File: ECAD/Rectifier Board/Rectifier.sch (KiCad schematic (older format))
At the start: 3 parts

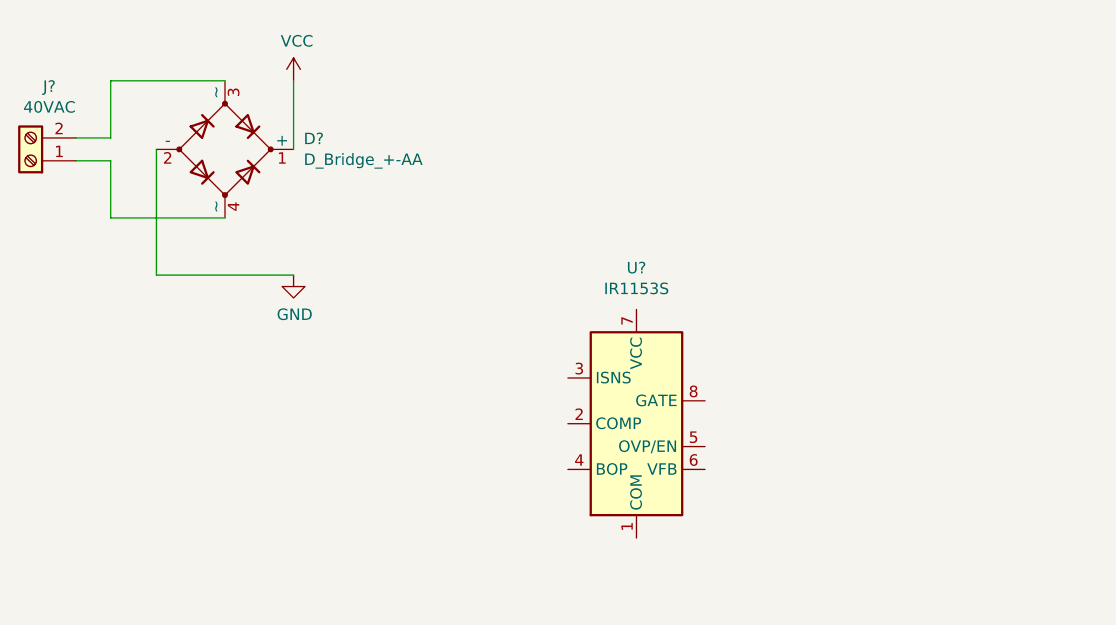
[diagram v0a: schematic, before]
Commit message: rectifier
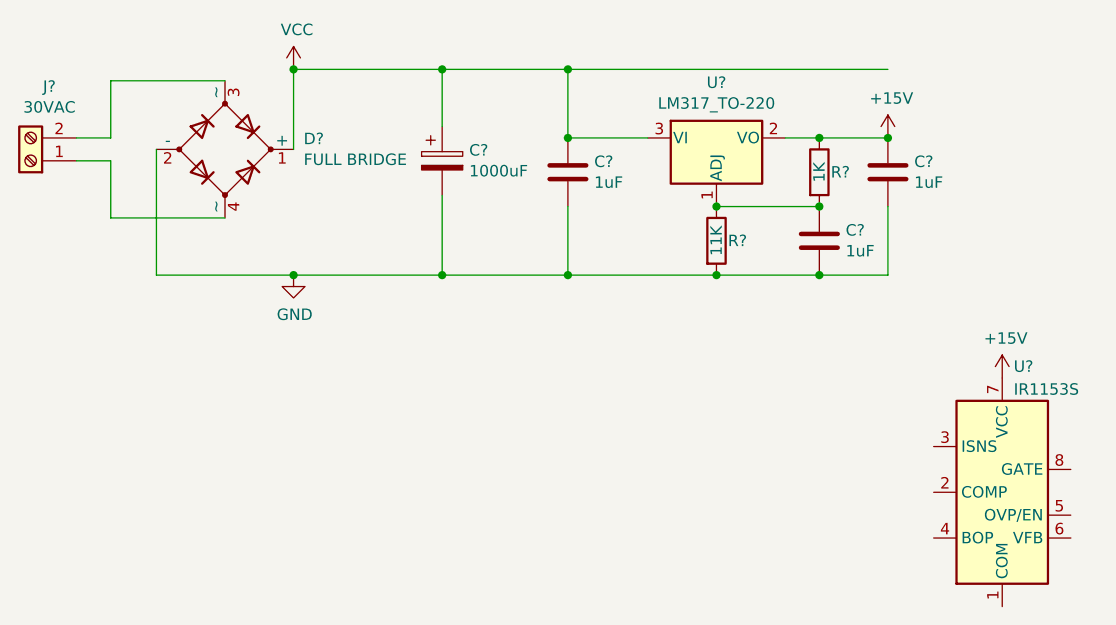
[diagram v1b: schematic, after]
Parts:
- added C? (x3): 1uF, symbol Device:C
- added C?: 1000uF, symbol Device:CP
- added R?: 11K, symbol Device:R
- added R?: 1K, symbol Device:R
- added U?: LM317_TO-220, Package_TO_SOT_THT:TO-220-3_Vertical, symbol Regulator_Linear:LM317_TO-220
- D?: value D_Bridge_+-AA -> FULL BRIDGE
- J?: value 40VAC -> 30VAC
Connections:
- net labels added: +15V
- wire segments 9 -> 26
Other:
- moved on the sheet: U?
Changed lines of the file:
@@
 P 3000 2950
 F 0 "D?" H 3344 2996 50  0000 L CNN
-F 1 "D_Bridge_+-AA" H 3344 2905 50  0000 L CNN
+F 1 "FULL BRIDGE" H 3344 2905 50  0000 L CNN
 F 2 "" H 3000 2950 50  0001 C CNN
 F 3 "~" H 3000 2950 50  0001 C CNN
@@
 L Regulator_Controller:IR1153S U?
 U 1 1 62058102
-P 4800 4150
-F 0 "U?" H 4800 4831 50  0000 C CNN
-F 1 "IR1153S" H 4800 4740 50  0000 C CNN
-F 2 "Package_SO:SOIC-8_3.9x4.9mm_P1.27mm" H 4800 4150 50  0001 C CIN
-F 3 "https://www.infineon.com/dgdl/ir1153.pdf?fileId=5546d462533600a4015355c42a5b1649" H 4800 4150 50  0001 C CNN
-	1    4800 4150
+P 6400 4450
+F 0 "U?" H 6450 5000 50  0000 L CNN
+F 1 "IR1153S" H 6450 4900 50  0000 L CNN
+F 2 "Package_SO:SOIC-8_3.9x4.9mm_P1.27mm" H 6400 4450 50  0001 C CIN
+F 3 "https://www.infineon.com/dgdl/ir1153.pdf?fileId=5546d462533600a4015355c42a5b1649" H 6400 4450 50  0001 C CNN
+	1    6400 4450
 	1    0    0    -1
 $EndComp
@@
 P 2150 3000
 F 0 "J?" H 2068 2675 50  0000 C CNN
-F 1 "40VAC" H 2068 2766 50  0000 C CNN
+F 1 "30VAC" H 2068 2766 50  0000 C CNN
 F 2 "" H 2150 3000 50  0001 C CNN
 F 3 "~" H 2150 3000 50  0001 C CNN
@@
 Wire Wire Line
 	2700 3500 3300 3500
-Wire Wire Line
-	3300 2950 3300 2650
 $Comp
 L power:VCC #PWR?
 U 1 1 6205AED4
-P 3300 2650
-F 0 "#PWR?" H 3300 2500 50  0001 C CNN
-F 1 "VCC" H 3315 2823 50  0000 C CNN
-F 2 "" H 3300 2650 50  0001 C CNN
-F 3 "" H 3300 2650 50  0001 C CNN
-	1    3300 2650
-	1    0    0    -1
-$EndComp
+P 3300 2600
+F 0 "#PWR?" H 3300 2450 50  0001 C CNN
+F 1 "VCC" H 3315 2773 50  0000 C CNN
+F 2 "" H 3300 2600 50  0001 C CNN
+F 3 "" H 3300 2600 50  0001 C CNN
+	1    3300 2600
+	1    0    0    -1
+$EndComp
+$Comp
+L Regulator_Linear:LM317_TO-220 U?
+U 1 1 6205D4E8
+P 5150 2900
+F 0 "U?" H 5150 3142 50  0000 C CNN
+F 1 "LM317_TO-220" H 5150 3051 50  0000 C CNN
+F 2 "Package_TO_SOT_THT:TO-220-3_Vertical" H 5150 3150 50  0001 C CIN
+F 3 "http://www.ti.com/lit/ds/symlink/lm317.pdf" H 5150 2900 50  0001 C CNN
+	1    5150 2900
+	1    0    0    -1
+$EndComp
+$Comp
+L Device:R R?
+U 1 1 6205E083
+P 5150 3350
+F 0 "R?" H 5200 3350 50  0000 L CNN
+F 1 "11K" V 5150 3350 50  0000 C CNN
+F 2 "" V 5080 3350 50  0001 C CNN
+F 3 "~" H 5150 3350 50  0001 C CNN
+	1    5150 3350
+	1    0    0    -1
+$EndComp
+$Comp
+L Device:R R?
+U 1 1 6205F378
+P 5600 3050
+F 0 "R?" H 5650 3050 50  0000 L CNN
+F 1 "1K" V 5600 3050 50  0000 C CNN
+F 2 "" V 5530 3050 50  0001 C CNN
+F 3 "~" H 5600 3050 50  0001 C CNN
+	1    5600 3050
+	1    0    0    -1
+$EndComp
+Wire Wire Line
+	5150 3200 5600 3200
+Connection ~ 5150 3200
+Wire Wire Line
+	5600 2900 5450 2900
+$Comp
+L Device:C C?
+U 1 1 6205FE8A
+P 5900 3050
+F 0 "C?" H 6015 3096 50  0000 L CNN
+F 1 "1uF" H 6015 3005 50  0000 L CNN
+F 2 "" H 5938 2900 50  0001 C CNN
+F 3 "~" H 5900 3050 50  0001 C CNN
+	1    5900 3050
+	1    0    0    -1
+$EndComp
+$Comp
+L Device:C C?
+U 1 1 620613FC
+P 5600 3350
+F 0 "C?" H 5715 3396 50  0000 L CNN
+F 1 "1uF" H 5715 3305 50  0000 L CNN
+F 2 "" H 5638 3200 50  0001 C CNN
+F 3 "~" H 5600 3350 50  0001 C CNN
+	1    5600 3350
+	1    0    0    -1
+$EndComp
+Connection ~ 5600 3200
+Wire Wire Line
+	5150 3500 5600 3500
+Wire Wire Line
+	5600 3500 5900 3500
+Wire Wire Line
+	5900 3500 5900 3200
+Connection ~ 5600 3500
+Wire Wire Line
+	5900 2900 5600 2900
+Connection ~ 5600 2900
+$Comp
+L Device:C C?
+U 1 1 620625CD
+P 4500 3050
+F 0 "C?" H 4615 3096 50  0000 L CNN
+F 1 "1uF" H 4615 3005 50  0000 L CNN
+F 2 "" H 4538 2900 50  0001 C CNN
+F 3 "~" H 4500 3050 50  0001 C CNN
+	1    4500 3050
+	1    0    0    -1
+$EndComp
+Wire Wire Line
+	4500 3500 4500 3200
+Wire Wire Line
+	4850 2900 4500 2900
+Wire Wire Line
+	4500 3500 5150 3500
+Connection ~ 5150 3500
+$Comp
+L Device:CP C?
+U 1 1 62063BAE
+P 3950 3000
+F 0 "C?" H 4068 3046 50  0000 L CNN
+F 1 "1000uF" H 4068 2955 50  0000 L CNN
+F 2 "" H 3988 2850 50  0001 C CNN
+F 3 "~" H 3950 3000 50  0001 C CNN
+	1    3950 3000
+	1    0    0    -1
+$EndComp
+Wire Wire Line
+	3300 2600 3950 2600
+Connection ~ 3300 2600
+Wire Wire Line
+	3300 3500 3950 3500
+Wire Wire Line
+	3950 3500 3950 3150
+Connection ~ 3300 3500
+Wire Wire Line
+	3950 2600 4500 2600
+Connection ~ 3950 2600
+Wire Wire Line
+	4500 2900 4500 2600
+Connection ~ 4500 2900
+Connection ~ 4500 2600
+Wire Wire Line
+	4500 2600 5900 2600
+Wire Wire Line
+	3950 2600 3950 2850
+Wire Wire Line
+	3300 2600 3300 2950
+Wire Wire Line
+	3950 3500 4500 3500
+Connection ~ 3950 3500
+Connection ~ 4500 3500
+$Comp
+L power:+15V #PWR?
+U 1 1 6206D11A
+P 5900 2900
+F 0 "#PWR?" H 5900 2750 50  0001 C CNN
+F 1 "+15V" H 5915 3073 50  0000 C CNN
+F 2 "" H 5900 2900 50  0001 C CNN
+F 3 "" H 5900 2900 50  0001 C CNN
+	1    5900 2900
+	1    0    0    -1
+$EndComp
+Connection ~ 5900 2900
+$Comp
+L power:+15V #PWR?
+U 1 1 6206D895
+P 6400 3950
+F 0 "#PWR?" H 6400 3800 50  0001 C CNN
+F 1 "+15V" H 6415 4123 50  0000 C CNN
+F 2 "" H 6400 3950 50  0001 C CNN
+F 3 "" H 6400 3950 50  0001 C CNN
+	1    6400 3950
+	1    0    0    -1
+$EndComp
